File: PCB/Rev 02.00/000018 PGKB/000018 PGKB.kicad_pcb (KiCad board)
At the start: 2 copper layers, 64.9 x 50.6 mm, 49 parts, among them J1 USB_B_V_Adam_USB-B-S-VT, U1 MCP1825T-3302E/DC, U2 CAT811TTBI-GT3, U3 RP2040, Y1 8 MHz

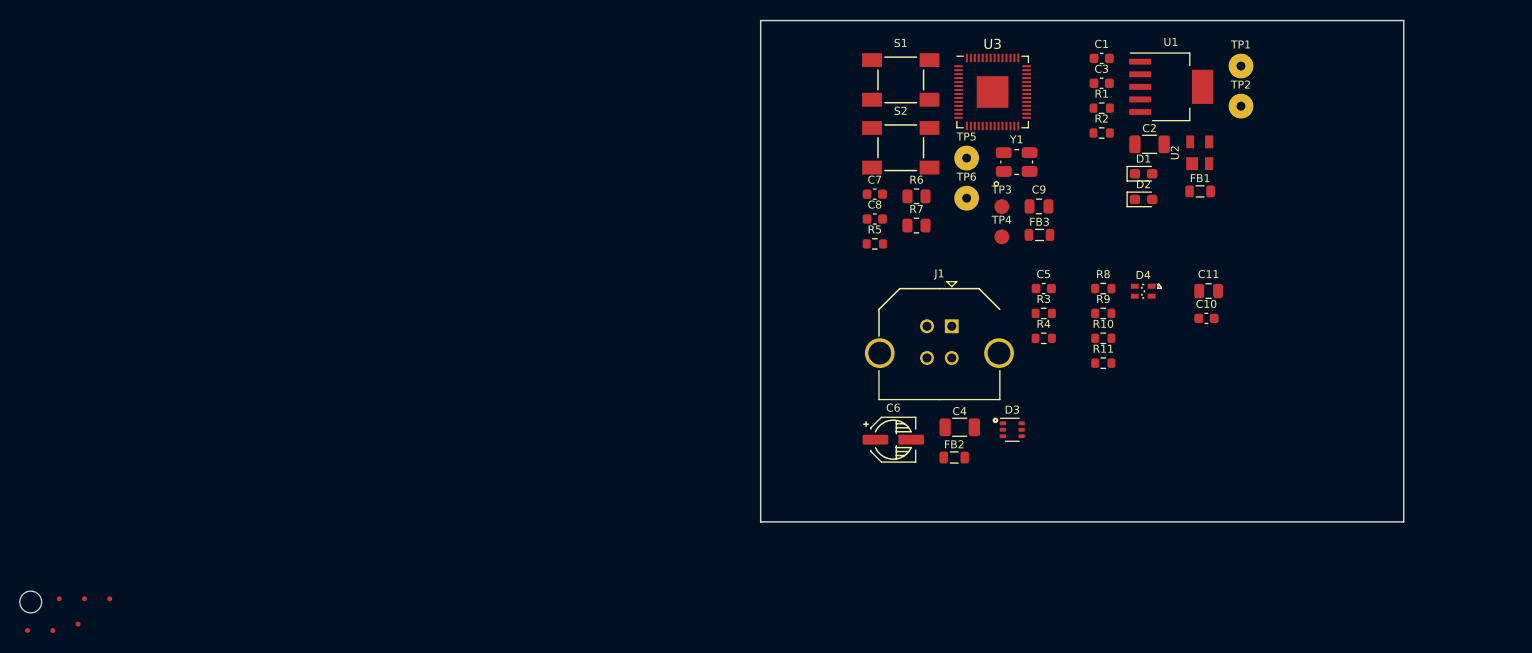
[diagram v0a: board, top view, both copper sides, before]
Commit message: schematic
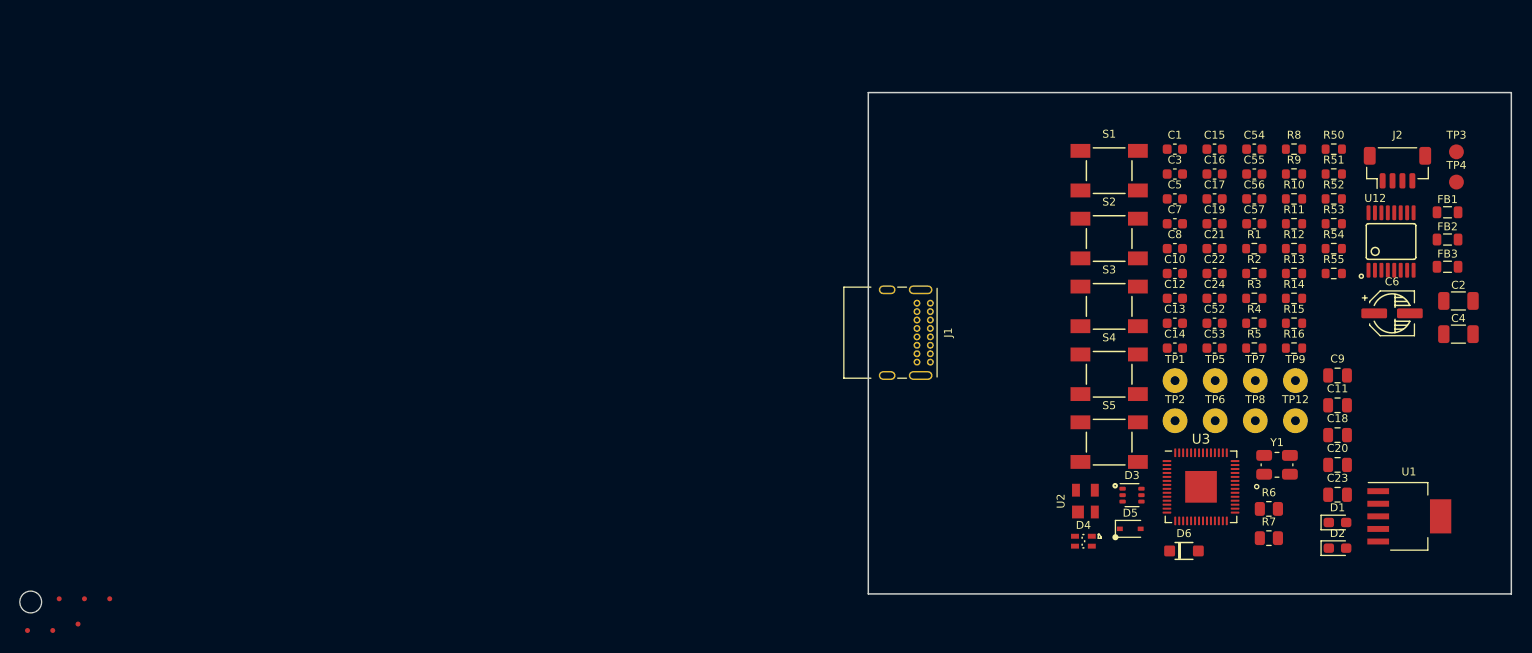
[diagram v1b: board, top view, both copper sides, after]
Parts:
- added C12: 27p, KD_Capacitor:CAPC1608X90N, F.Cu at (170.4, 103.4)
- added C13: 100n, KD_Capacitor:CAPC1608X90N, F.Cu at (170.4, 106.0)
- added C14: 100n, KD_Capacitor:CAPC1608X90N, F.Cu at (170.4, 108.5)
- added C15: 100n, KD_Capacitor:CAPC1608X90N, F.Cu at (174.4, 88.4)
- added C16: 100n, KD_Capacitor:CAPC1608X90N, F.Cu at (174.4, 90.9)
- added C17: 100n, KD_Capacitor:CAPC1608X90N, F.Cu at (174.4, 93.4)
- added C18: 1u, KD_Capacitor:CAPC2012X135N, F.Cu at (186.8, 117.2)
- added C19: 100n, KD_Capacitor:CAPC1608X90N, F.Cu at (174.4, 95.9)
- added C20: 1u, KD_Capacitor:CAPC2012X135N, F.Cu at (186.8, 120.2)
- added C21: 100n, KD_Capacitor:CAPC1608X90N, F.Cu at (174.4, 98.4)
- added C22: 100n, KD_Capacitor:CAPC1608X90N, F.Cu at (174.4, 100.9)
- added C23: 1u, KD_Capacitor:CAPC2012X135N, F.Cu at (186.8, 123.3)
- added C24: 100n, KD_Capacitor:CAPC1608X90N, F.Cu at (174.4, 103.4)
- added C52: 10n, KD_Capacitor:CAPC1608X90N, F.Cu at (174.4, 106.0)
- added C53: 10n, KD_Capacitor:CAPC1608X90N, F.Cu at (174.4, 108.5)
- added C54: 10n, KD_Capacitor:CAPC1608X90N, F.Cu at (178.4, 88.4)
- added C55: 10n, KD_Capacitor:CAPC1608X90N, F.Cu at (178.4, 90.9)
- added C56: 10n, KD_Capacitor:CAPC1608X90N, F.Cu at (178.4, 93.4)
- added C57: 10n, KD_Capacitor:CAPC1608X90N, F.Cu at (178.4, 95.9)
- added D5: Schottky_30V_200mA_DCo_BAT54WS, KD_Diode:D_SOD-323, F.Cu at (165.9, 126.7)
- added D6: Schottky_30V_1A_PMEG3010ER_115, KD_Diode:DIOC360X180X150_SOD123, F.Cu at (171.3, 128.9)
- added J2: BM04B-SRSS-TB, KD_Connector_Rectangular:JST_SH_BM04B-SRSS-TB_1x04-1MP_P1.00mm_Vertical, F.Cu at (192.9, 90.2)
- added R12: 1k, KD_Resistor:RESC1608X55N, F.Cu at (182.4, 98.4)
- added R13: 1k, KD_Resistor:RESC1608X55N, F.Cu at (182.4, 100.9)
- added R14: R_0603_5100_1%, KD_Resistor:RESC1608X55N, F.Cu at (182.4, 103.4)
- added R15: R_0603_5100_1%, KD_Resistor:RESC1608X55N, F.Cu at (182.4, 106.0)
- added R16: 10k, KD_Resistor:RESC1608X55N, F.Cu at (182.4, 108.5)
- added R50: 1k, KD_Resistor:RESC1608X55N, F.Cu at (186.4, 88.4)
- added R51: 1k, KD_Resistor:RESC1608X55N, F.Cu at (186.4, 90.9)
- added R52: 1k, KD_Resistor:RESC1608X55N, F.Cu at (186.4, 93.4)
- added R53: 1k, KD_Resistor:RESC1608X55N, F.Cu at (186.4, 95.9)
- added R54: 1k, KD_Resistor:RESC1608X55N, F.Cu at (186.4, 98.4)
- added R55: 1k, KD_Resistor:RESC1608X55N, F.Cu at (186.4, 100.9)
- added S3: Button_tactile_45x38_430181038816, KD_Switch:SW_Push_1P1T_NO_Wurth_430181038816, F.Cu at (163.8, 104.2)
- added S4: Button_tactile_45x38_430181038816, KD_Switch:SW_Push_1P1T_NO_Wurth_430181038816, F.Cu at (163.8, 111.1)
- added S5: Button_tactile_45x38_430181038816, KD_Switch:SW_Push_1P1T_NO_Wurth_430181038816, F.Cu at (163.8, 118.0)
- added TP12: TP D2.5 mm H0.9mm, KD_Connector_Pads:TestPoint_Pad_D2.5mm_H0.9mm, F.Cu at (182.6, 115.8)
- added TP7: TP D2.5 mm H0.9mm, KD_Connector_Pads:TestPoint_Pad_D2.5mm_H0.9mm, F.Cu at (178.5, 111.7)
- added TP8: TP D2.5 mm H0.9mm, KD_Connector_Pads:TestPoint_Pad_D2.5mm_H0.9mm, F.Cu at (178.5, 115.8)
- added TP9: TP D2.5 mm H0.9mm, KD_Connector_Pads:TestPoint_Pad_D2.5mm_H0.9mm, F.Cu at (182.6, 111.7)
- added U12: SN74HCS365PWR, KD_Package_SO:SOP65P600X150-16N, F.Cu at (192.2, 97.7)
- C7: value 100n -> 27p
- J1: value USB_B_V_Adam_USB-B-S-VT -> USB Mini B; footprint KD_Connector_USB_HDMI_Etc:USB_B_Vertical_Adam_USB-B-S-VT -> KD_Connector_USB_HDMI_Etc:USB_C_Receptacle_GCT_USB4085
- R5: footprint KD_Resistor:RESC1608X55N -> KD_Resistor:RESC1608X55N_DNP
- Y1: value 8 MHz -> 12 MHz
- moved FB2 54.4 mm to (197.9, 97.5)
- moved C6 51.9 mm to (192.3, 105.0)
- moved C4 51.2 mm to (199.0, 107.0)
- moved U1 49.6 mm to (194.1, 125.4)
- moved R6 47.5 mm to (179.9, 124.7)
- moved R7 47.5 mm to (179.9, 127.6)
- moved TP3 46.2 mm to (198.8, 88.7)
- moved TP4 46.2 mm to (198.8, 91.7)
- moved U3 45.1 mm to (173.0, 122.5)
- moved FB3 41.3 mm to (197.9, 100.2)
- moved Y1 40.3 mm to (180.7, 120.2)
- moved D1 40.3 mm to (186.8, 126.1)
- moved D2 40.3 mm to (186.8, 128.7)
- moved R5 39.7 mm to (178.4, 108.5)
- moved U2 37.0 mm to (161.4, 123.9)
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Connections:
- C7 pad 1: GND -> Net-(U3-XIN)
- C7 pad 2: +3V3 -> GND
- C8 pad 1: Net-(C8-Pad1) -> Net-(U3-ADC_AVDD)
- C9 pad 1: Net-(C8-Pad1) -> Net-(U3-ADC_AVDD)
- FB2 pad 1: Net-(D3-V+) -> Net-(D6-K)
- FB3 pad 1: unconnected-(FB3-Pad1) -> +3V3
- FB3 pad 2: unconnected-(FB3-Pad2) -> Net-(U3-ADC_AVDD)
- R6 pad 2: /Main/Microcontroller/SCL -> /Main/Microcontroller/SDA
- R7 pad 2: /Main/Microcontroller/SDA -> /Main/Microcontroller/SCL
- S2 pad 3: /Main/Microcontroller/BOOT -> /Main/Microcontroller/USBBOOT
- TP5 pad 1: /Main/Microcontroller/SDA -> /Main/Microcontroller/SCL
- TP6 pad 1: /Main/Microcontroller/SCL -> /Main/Microcontroller/SDA
- U3 pad 1: Net-(U3-IOVDD-Pad1) -> Net-(U3-ADC_AVDD)
- U3 pad 10: Net-(U3-IOVDD-Pad1) -> Net-(U3-ADC_AVDD)
- U3 pad 19: unconnected-(U3-TESTEN-Pad19) -> GND
- U3 pad 2: unconnected-(U3-GPIO0-Pad2) -> /Main/Microcontroller/GPIO0
- U3 pad 21: unconnected-(U3-XOUT-Pad21) -> Net-(U3-XOUT)
- U3 pad 22: Net-(U3-IOVDD-Pad1) -> Net-(U3-ADC_AVDD)
- U3 pad 23: Net-(U3-DVDD-Pad23) -> /Main/Microcontroller/1V2
- U3 pad 3: unconnected-(U3-GPIO1-Pad3) -> /Main/Microcontroller/GPIO1
- U3 pad 30: unconnected-(U3-GPIO19-Pad30) -> /Main/Microcontroller/UART_TX
- U3 pad 32: unconnected-(U3-GPIO21-Pad32) -> /Main/Microcontroller/USBBOOT
- U3 pad 33: Net-(U3-IOVDD-Pad1) -> Net-(U3-ADC_AVDD)
- U3 pad 34: unconnected-(U3-GPIO22-Pad34) -> /Main/Microcontroller/I2C1_SDA
- U3 pad 35: unconnected-(U3-GPIO23-Pad35) -> /Main/Microcontroller/I2C1_SCL
- U3 pad 36: unconnected-(U3-GPIO24-Pad36) -> /Main/Microcontroller/SDA
- U3 pad 37: unconnected-(U3-GPIO25-Pad37) -> /Main/Microcontroller/SCL
- U3 pad 4: unconnected-(U3-GPIO2-Pad4) -> /Main/Microcontroller/GPIO2
- U3 pad 42: Net-(U3-IOVDD-Pad1) -> Net-(U3-ADC_AVDD)
- U3 pad 43: unconnected-(U3-ADC_AVDD-Pad43) -> Net-(U3-ADC_AVDD)
- U3 pad 44: unconnected-(U3-VREG_IN-Pad44) -> Net-(U3-ADC_AVDD)
- U3 pad 45: unconnected-(U3-VREG_VOUT-Pad45) -> /Main/Microcontroller/1V2
- U3 pad 48: unconnected-(U3-USB_VDD-Pad48) -> Net-(U3-ADC_AVDD)
- U3 pad 49: Net-(U3-IOVDD-Pad1) -> Net-(U3-ADC_AVDD)
- U3 pad 5: unconnected-(U3-GPIO3-Pad5) -> /Main/Microcontroller/SPI_MOSI
- U3 pad 50: Net-(U3-DVDD-Pad23) -> /Main/Microcontroller/1V2
- U3 pad 6: unconnected-(U3-GPIO4-Pad6) -> /Main/Microcontroller/SPI_MISO
- U3 pad 7: unconnected-(U3-GPIO5-Pad7) -> /Main/Microcontroller/UART_RX
- U3 pad 8: unconnected-(U3-GPIO6-Pad8) -> /Main/Microcontroller/SPI_CLK
- Y1 pad 1: +3V3 -> Net-(U3-XIN)
- Y1 pad 3: Net-(U3-XIN) -> Net-(C12-Pad1)
- Y1 pad 4: +3V3 -> GND
